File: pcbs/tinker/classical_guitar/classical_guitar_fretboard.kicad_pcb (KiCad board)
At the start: 4 copper layers, 188 parts, among them Q1 AO3401A, U1 AT42QT1110-A, U2 AT42QT1110-A, U3 AT42QT1110-A, U4 MP2359

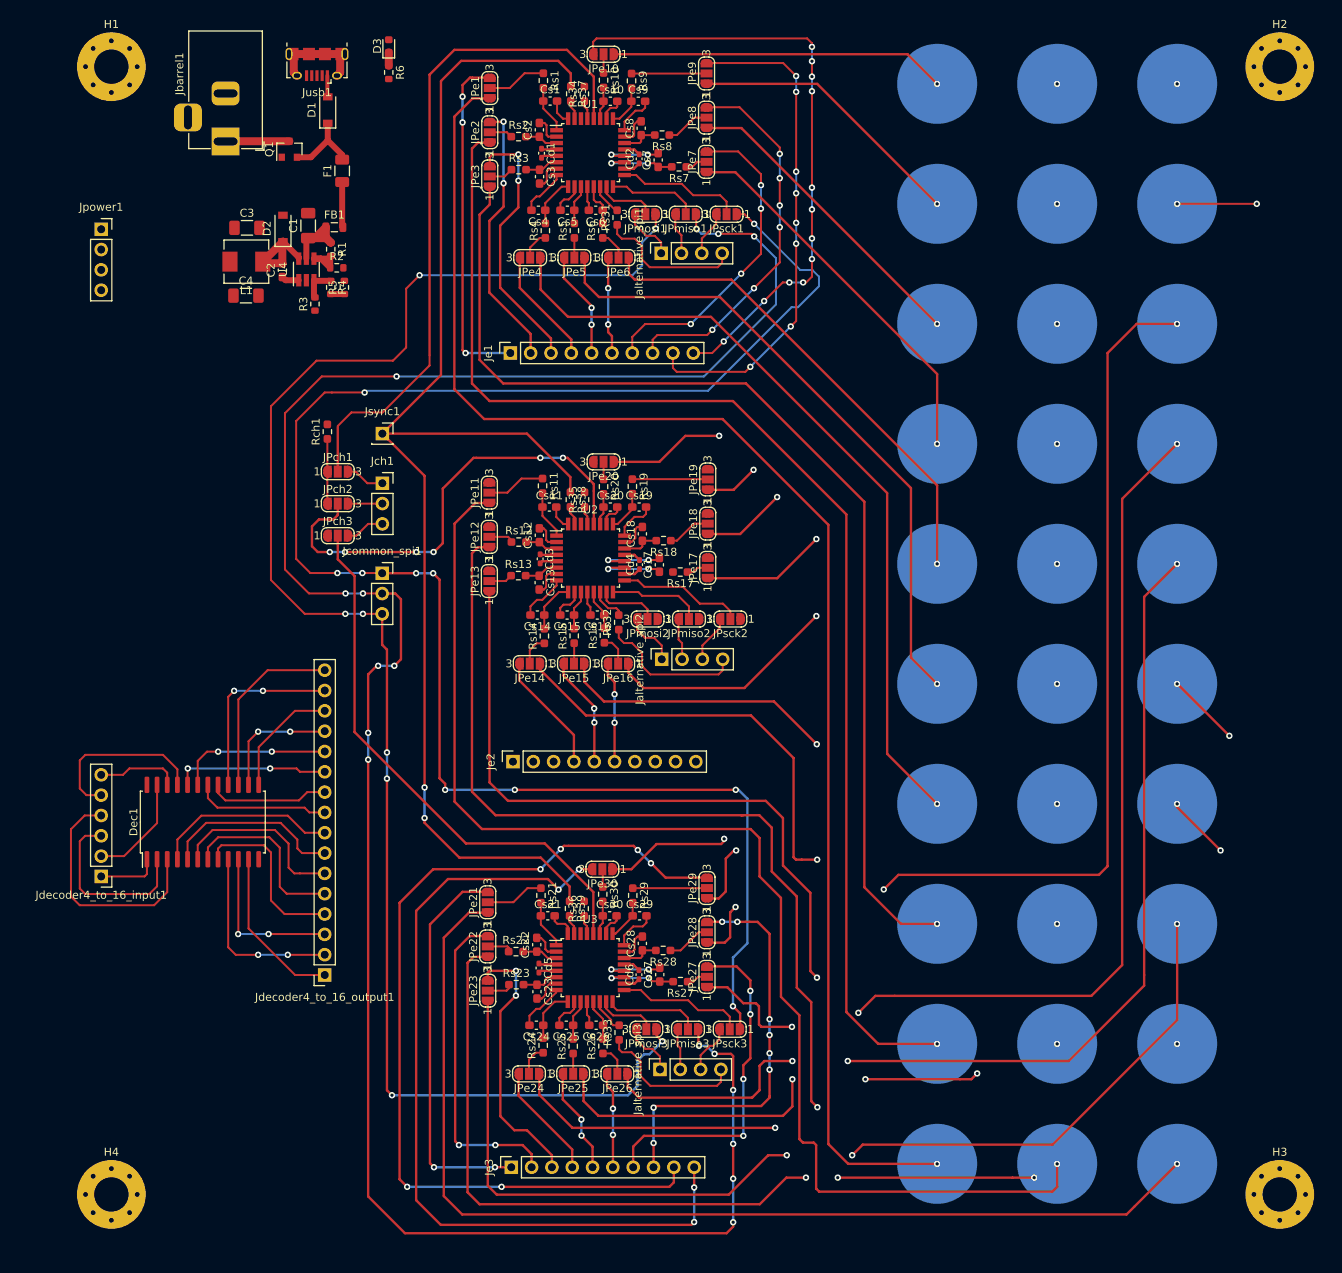
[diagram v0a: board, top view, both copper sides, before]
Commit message: Almost finalized pcb
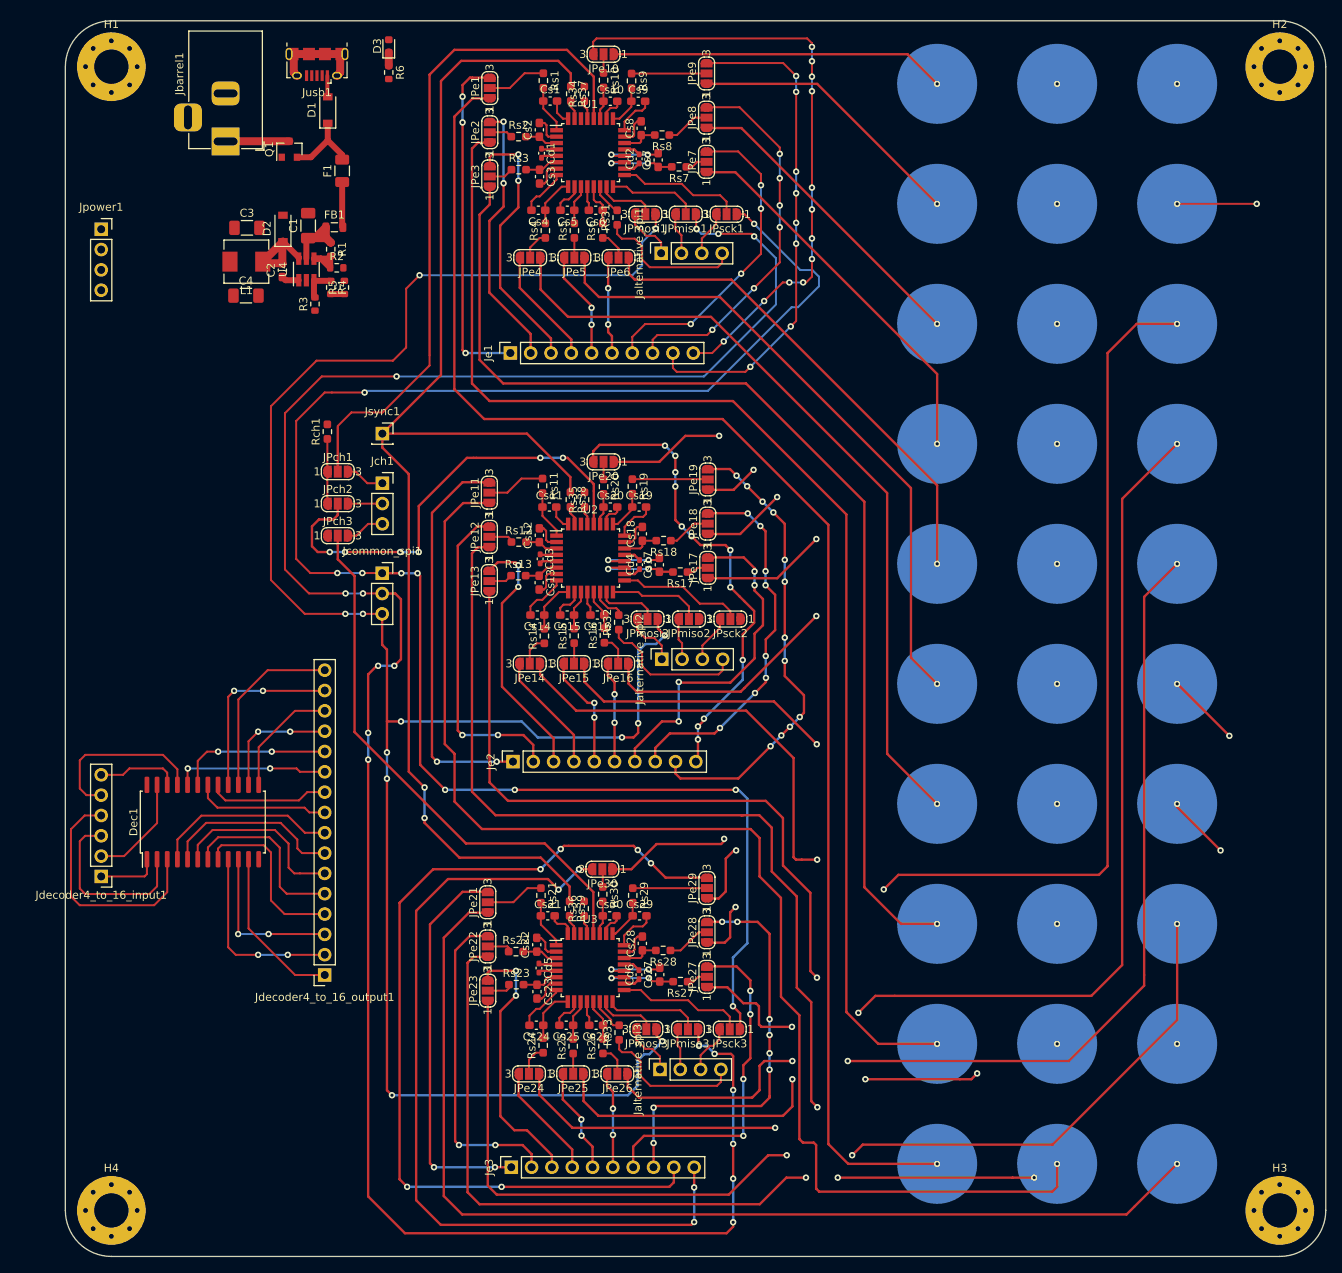
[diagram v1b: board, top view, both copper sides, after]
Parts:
- moved H3 2.00 mm to (177.8, 160.8)
- moved H4 2.00 mm to (31.8, 160.8)
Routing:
- net Net-(JPe20-Pad3): track 0.00 -> 59.7 mm, vias 0 -> 12
- net Net-(JPe19-Pad3): track 0.00 -> 58.3 mm, vias 0 -> 12
- net Net-(JPe11-Pad3): track 0.00 -> 49.6 mm, vias 0 -> 2
- net /C_MOSI: track 203.4 -> 252.6 mm, vias 8 -> 12
- net Net-(JPe18-Pad3): track 0.00 -> 47.0 mm, vias 0 -> 8
- net Net-(JPe17-Pad3): track 0.00 -> 42.8 mm, vias 0 -> 4
- net Net-(JPe12-Pad3): track 0.00 -> 40.3 mm, vias 0 -> 2
- net Net-(JPe13-Pad3): track 0.00 -> 32.3 mm, vias 0 -> 2
- net Net-(E11-Pad1): track 161.1 -> 163.0 mm
- net Net-(Cs17-Pad1): track 8.66 -> 10.4 mm
- net Net-(E16-Pad1): track 62.0 -> 63.1 mm
- net /C_SCK: track 218.0 -> 216.8 mm
- net /Change2: track 58.5 -> 57.8 mm
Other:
- board outline added: 157.6 x 154.4 mm
